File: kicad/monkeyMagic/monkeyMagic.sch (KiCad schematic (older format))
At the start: 67 parts, among them IC3 74LS03

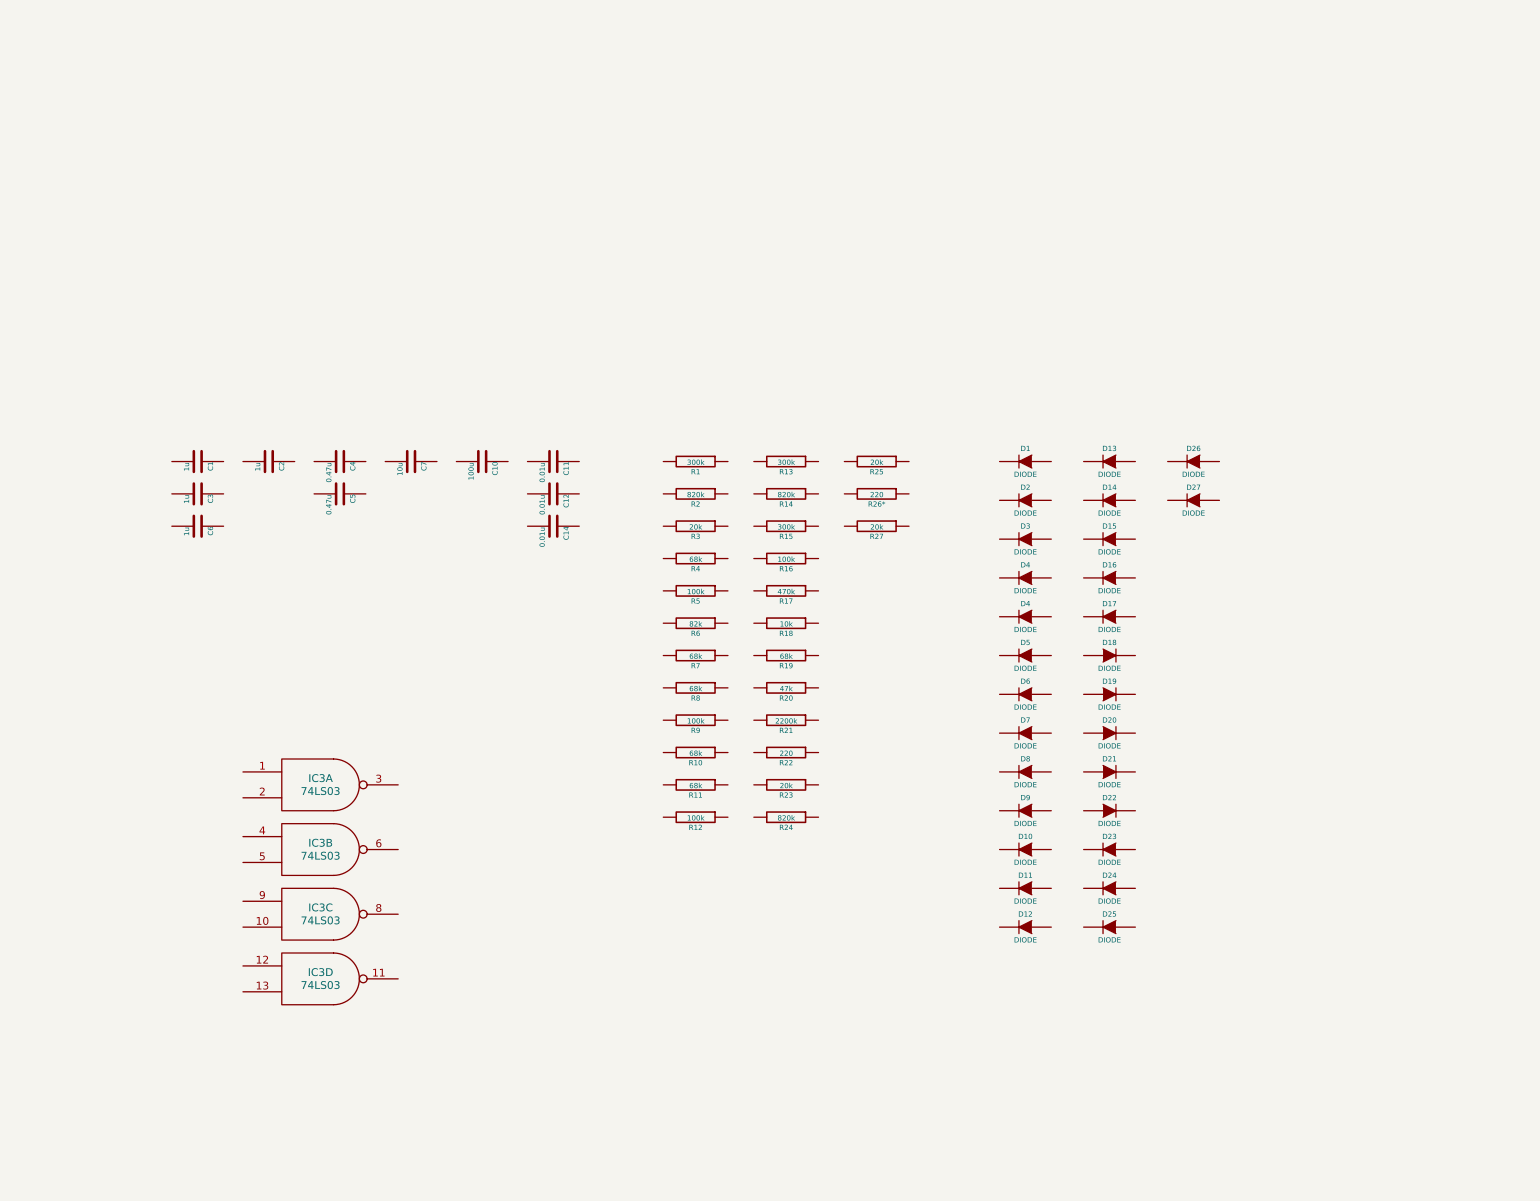
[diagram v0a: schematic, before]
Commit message: A MAME part library is born & some further Monkey Magic work.
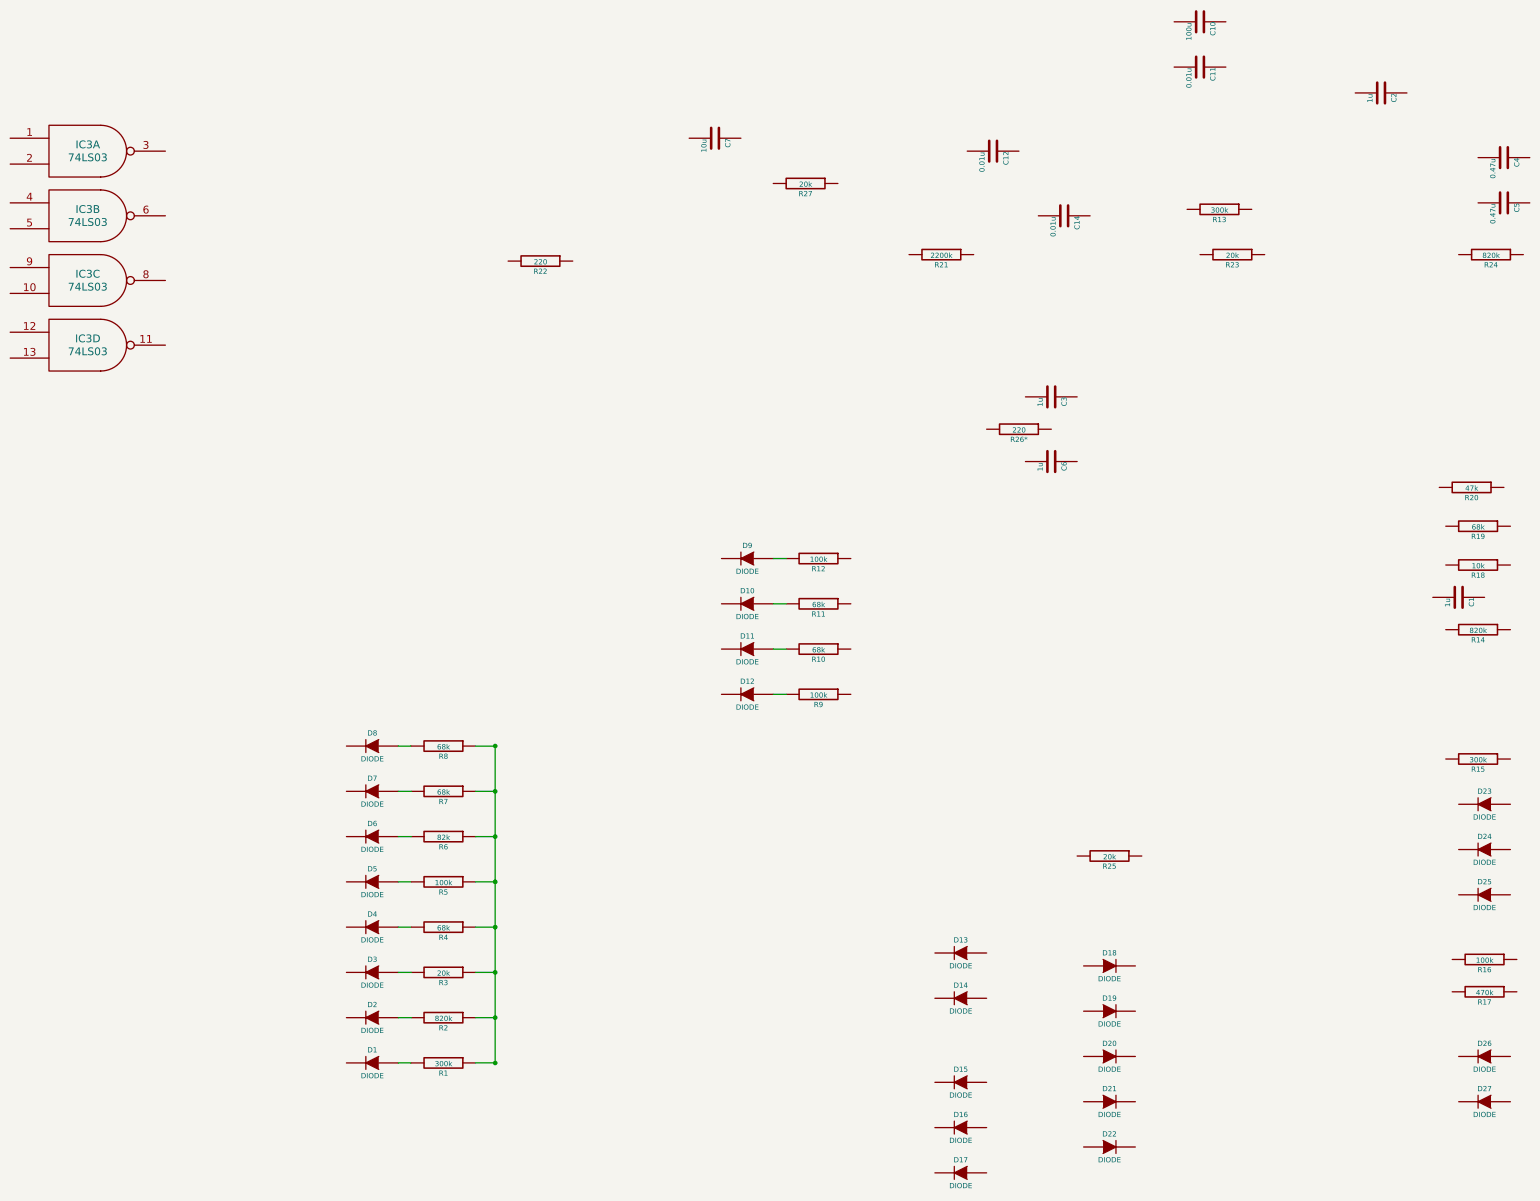
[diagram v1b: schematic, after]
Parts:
- removed D4: DIODE, ~, symbol DIODE
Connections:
- net at R1.1: now also R2.1, R3.1, R4.1, R5.1, R6.1, R7.1, R8.1
- net at R1.2: now also D1.1 (A)
- net at R2.2: now also D2.1 (A)
- net at R3.2: now also D3.1 (A)
- net at R4.2: now also D4.1 (A)
- net at R5.2: now also D5.1 (A)
- net at R6.2: now also D6.1 (A)
- net at R7.2: now also D7.1 (A)
- net at R8.2: now also D8.1 (A)
- net at R9.2: now also D12.1 (A)
- net at R10.2: now also D11.1 (A)
- net at R11.2: now also D10.1 (A)
- net at R12.2: now also D9.1 (A)
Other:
- moved on the sheet: C1, C10, C11, C12, C14, C2, C3, C4, C5, C6, C7, D1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

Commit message: Nearly fully-wired now.
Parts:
- added IC?: SN74123, ~, symbol SN74123
- added IC?: SN76477, ~, symbol SN76477
- added IC?: M53242, ~, symbol M53242
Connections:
- net labels added: GND, HELLO, VCC
- wire segments 21 -> 388
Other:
- note added: "Disconnected on our MMagic"
- note added: "Pin 14"
- note added: "Pin 7"
- note added: "Resistor Array"
- note added: "Resistor\nArray\nOf Some\nSort"
- note added: "Trace #1"
- note added: "Trace #10"
- note added: "Trace #11"
- note added: "Trace #12"
- note added: "Trace #13"
- note added: "Trace #14\n"
- note added: "Trace #15"
- note added: "Trace #16"
- note added: "Trace #17"
- note added: "Trace #18"
- note added: "Trace #2"
- note added: "Trace #21"
- note added: "Trace #22"
- note added: "Trace #23"
- note added: "Trace #25"
- note added: "Trace #26"
- note added: "Trace #27"
- note added: "Trace #28"
- note added: "Trace #3"
- note added: "Trace #31"
- note added: "Trace #32"
- note added: "Trace #33"
- note added: "Trace #34"
- note added: "Trace #35"
- note added: "Trace #36 ****"
- note added: "Trace #38"
- note added: "Trace #39"
- note added: "Trace #40"
- note added: "Trace #41"
- note added: "Trace #42"
- note added: "Trace #43"
- note added: "Trace #44\n"
- note added: "Trace #45\n"
- note added: "Trace #46\n"
- note added: "Trace #5"
- note added: "Trace #6"
- note added: "Trace #7"
- note added: "Trace #8"
- note added: "Trace #9"
- note added: "VR1?"
- moved on the sheet: C1, C10, C11, C12, C14, C2, C3, C4, C5, C6, C7, D1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
